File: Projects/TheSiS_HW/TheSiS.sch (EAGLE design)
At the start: 64 parts, among them IC1 REG1117, IC3 TP4056, IC4 MCP1703CB, IC5 CP2102, K1 G5L, K2 G5L, K3 G5L, T1 DMN3024LSD, U1 ESP-WROOM-32, U2 GY-521MPU6050, X2 ZX62D-B-5PA8

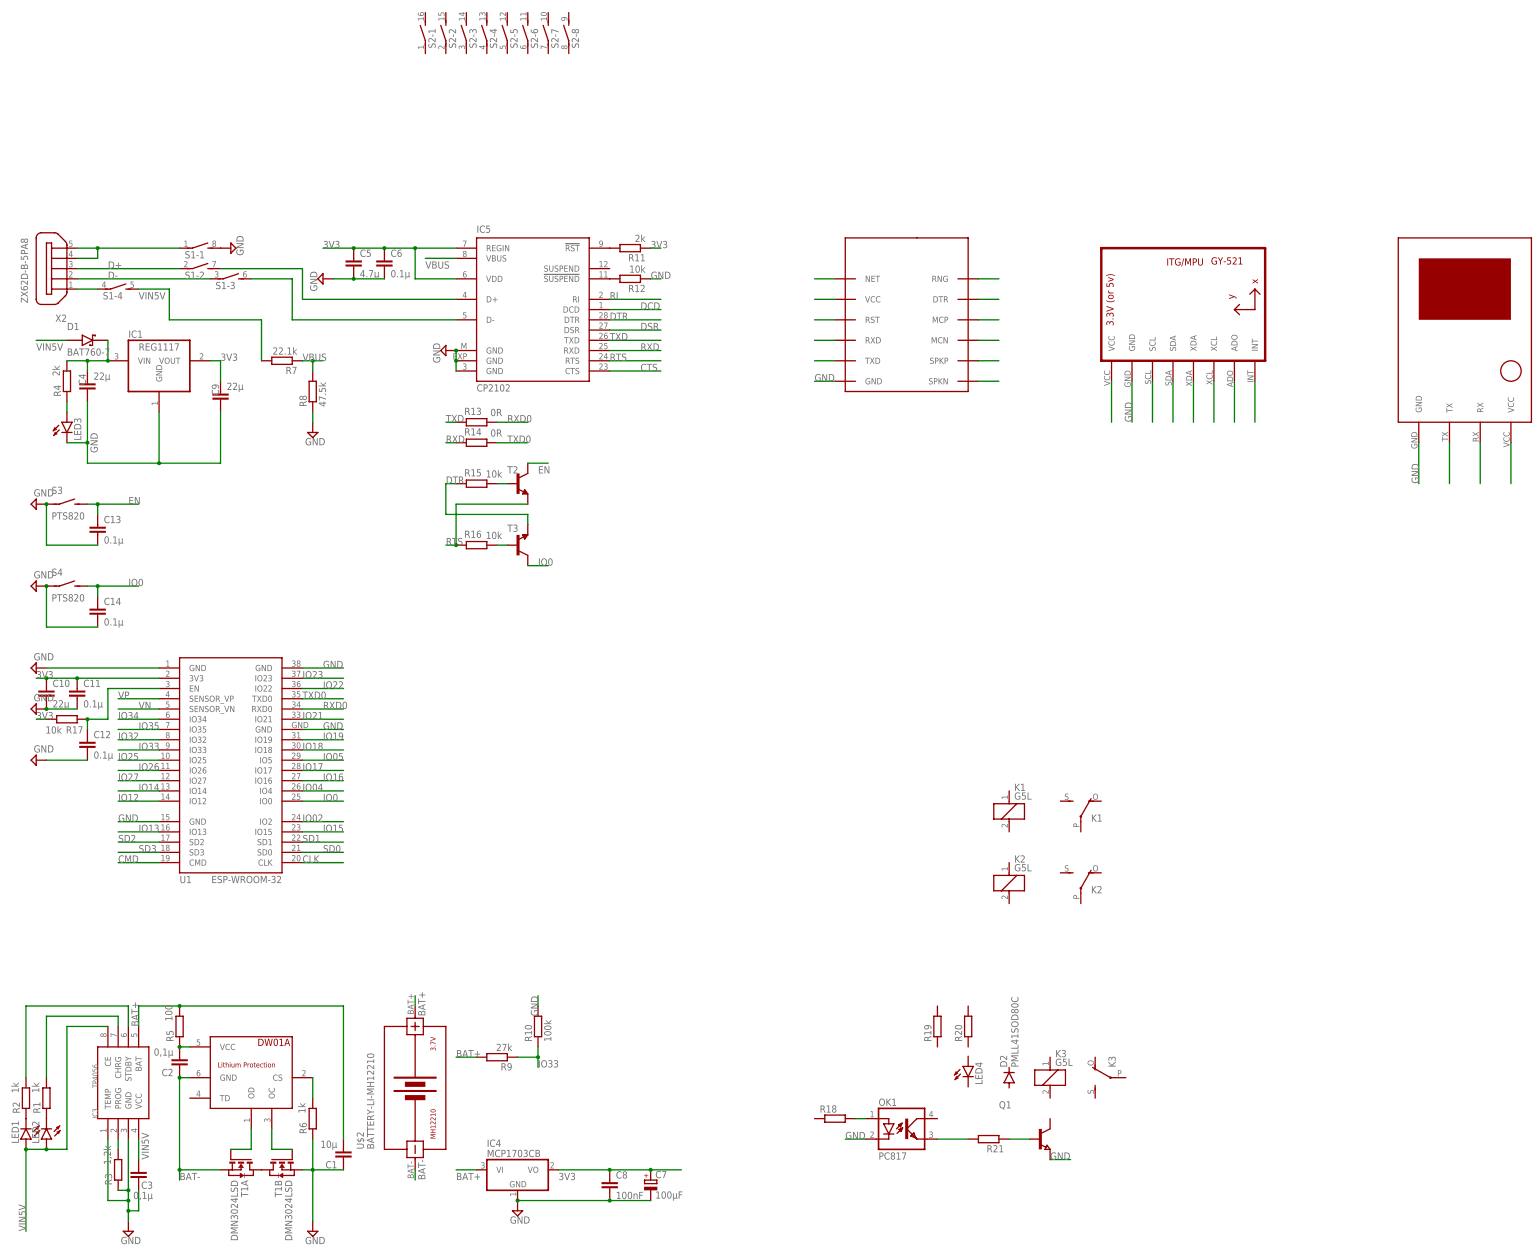
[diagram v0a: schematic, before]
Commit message: Finish TheSiS_HW Schematic
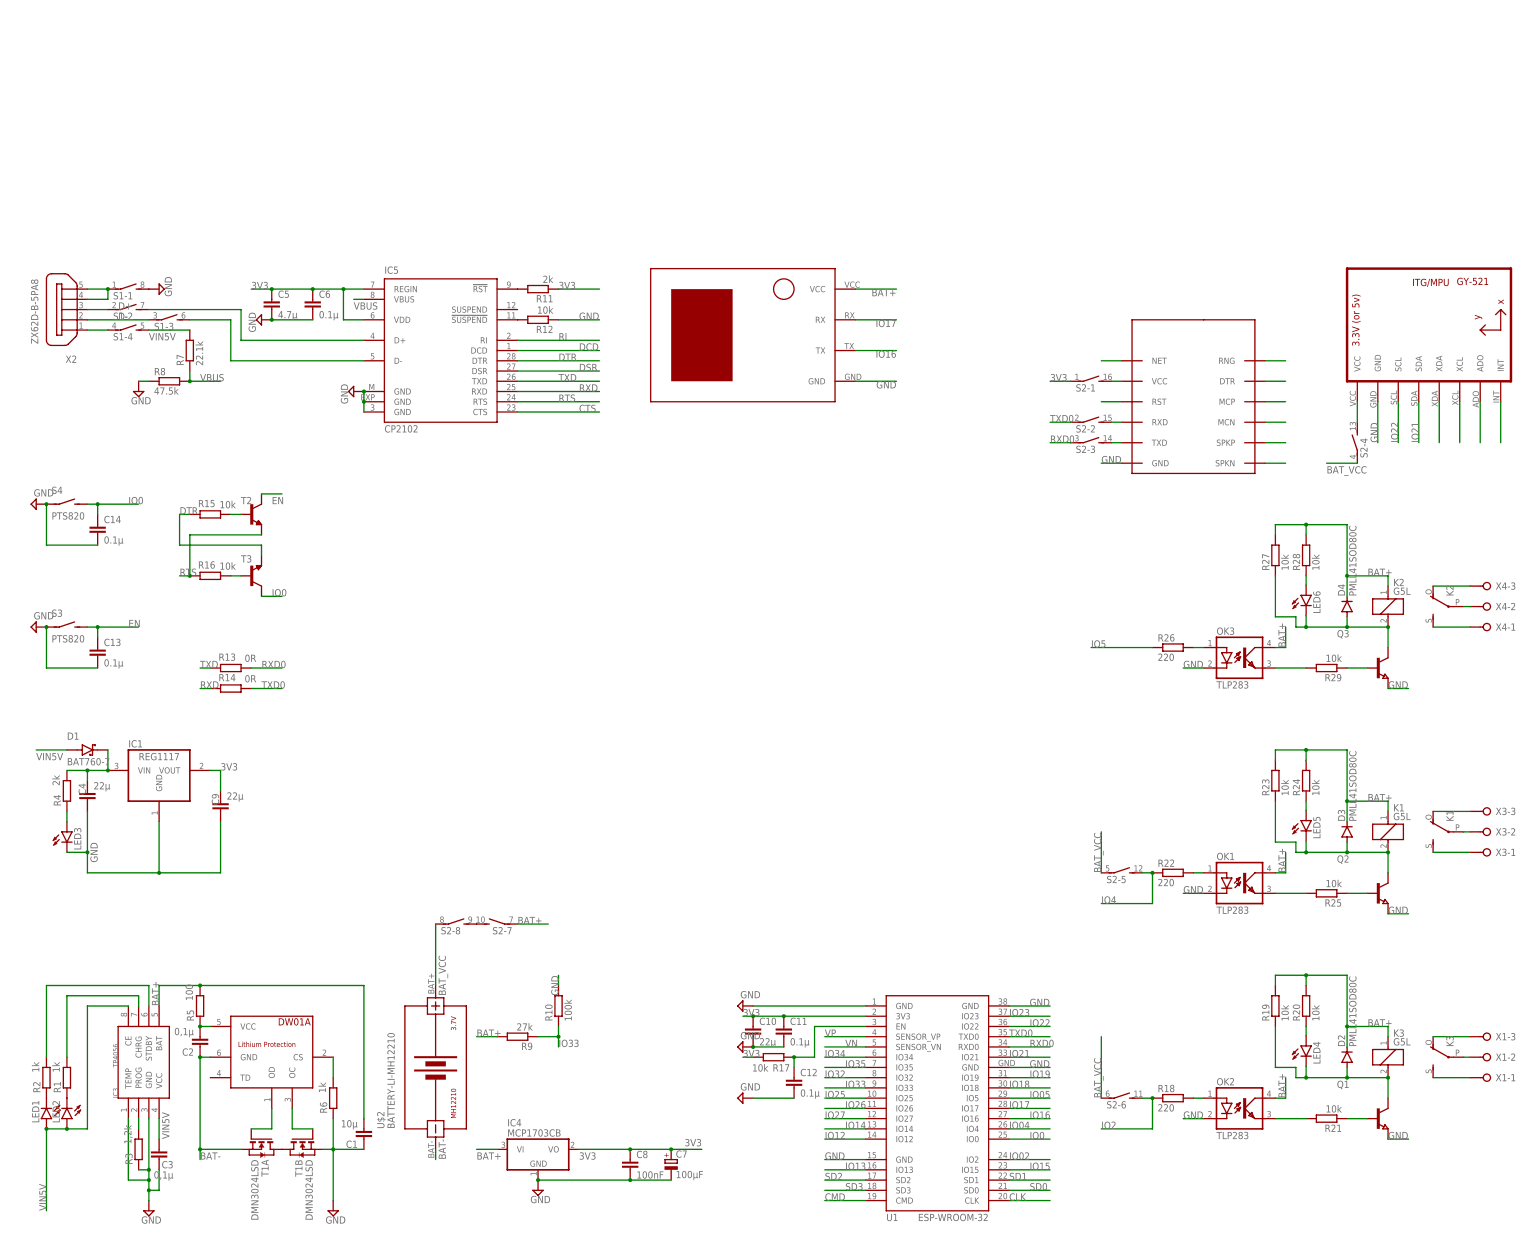
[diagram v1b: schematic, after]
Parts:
- added D3, D4: PMLL41SOD80C, diode:PMLL41SOD80C
- added LED5, LED6: (no value), led:LEDCHIP-LED0805
- added OK2, OK3: TLP283, optocoupler:TLP283
- added Q2, Q3: (no value), semicon-smd-ipc:NPN-TRANSISTOR_SOT23
- added R22, R26: 220, rcl:R-EU_R0805
- added R23, R24, R25, R27, R28, R29: 10k, rcl:R-EU_R0805
- added X1, X3, X4: (no value), con-wago-508:W237-03P
- OK1: value PC817 -> TLP283; device optocoupler:PC817 -> optocoupler:TLP283
- R18: value (none) -> 220
- R19, R20, R21: value (none) -> 10k
- T2, T3: SPICEPREFIX (none) -> J
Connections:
- removed net N$35: U2.SCL
- removed net N$36: U2.SDA
- new net $VCCSIM800: S2-1.2, U$4.VCC
- new net BAT_VCC: S2-4.1, S2-5.1, S2-6.1, S2-8.1, U$2.BAT+
- new net IO2: R18.1, S2-6.2
- new net IO4: R22.1, S2-5.2
- new net IO5: R26.1
- new net N$45: D2.A, K31.2, LED4.C, Q1.C, R19.1
- new net N$46: K32.O, X1-3.KL
- new net N$47: K32.P, X1-2.KL
- new net N$48: K32.S, X1-1.KL
- new net N$49: LED4.A, R20.1
- new net N$50: OK1.A, R22.2
- new net N$51: OK1.EMIT, R25.2
- new net N$52: Q2.B, R25.1
- new net N$53: D3.A, K11.2, LED5.C, Q2.C, R23.1
- new net N$54: LED5.A, R24.1
- new net N$55: K12.O, X3-3.KL
- new net N$56: K12.P, X3-2.KL
- new net N$57: K12.S, X3-1.KL
- new net N$58: D4.A, K21.2, LED6.C, Q3.C, R27.1
- new net N$59: LED6.A, R28.1
- new net N$60: K22.O, X4-3.KL
- new net N$61: K22.P, X4-2.KL
- new net N$62: K22.S, X4-1.KL
- net 3V3: now also S2-1.1
- net BAT+: now also D2.C, D3.C, D4.C, K11.1, K21.1, K31.1, OK1.COL, OK2.COL, OK3.COL, R19.2, R20.2, R23.2, R24.2, R27.2, R28.2, S2-7.1, U$3.VCC; no longer U$2.BAT+
- net GND: now also OK2.C, OK3.C, Q2.E, Q3.E
- net IO16: now also U$3.TX
- net IO17: now also U$3.RX
- net IO21: now also U2.SDA
- net IO22: now also U2.SCL
- net N$22: now also S2-7.2, S2-8.2; no longer U$4.VCC
- net N$24: now also S2-2.2
- net N$25: now also S2-3.2
- net N$26: now also OK2.A; no longer OK1.A
- net N$33: now also S2-4.2
- net N$34: now also OK2.EMIT; no longer OK1.EMIT
- net N$42: now also OK3.A, R26.2; no longer U$3.TX
- net N$43: now also OK3.EMIT, R29.2; no longer U$3.RX
- net N$44: now also Q3.B, R29.1; no longer U$3.VCC
- net RXD0: now also S2-3.1
- net TXD0: now also S2-2.1
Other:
- moved on the sheet: C1, C10, C11, C12, C13, C14, C2, C3, C4, C5, C6, C7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
